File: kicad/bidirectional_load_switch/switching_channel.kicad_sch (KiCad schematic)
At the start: 17 parts, among them U201 SN74LVC1G08DCKR, U202 SN74LVC1G17DCKR, U203 UCC23313DWYR, U204 STD16N60M6, U205 STD16N60M6

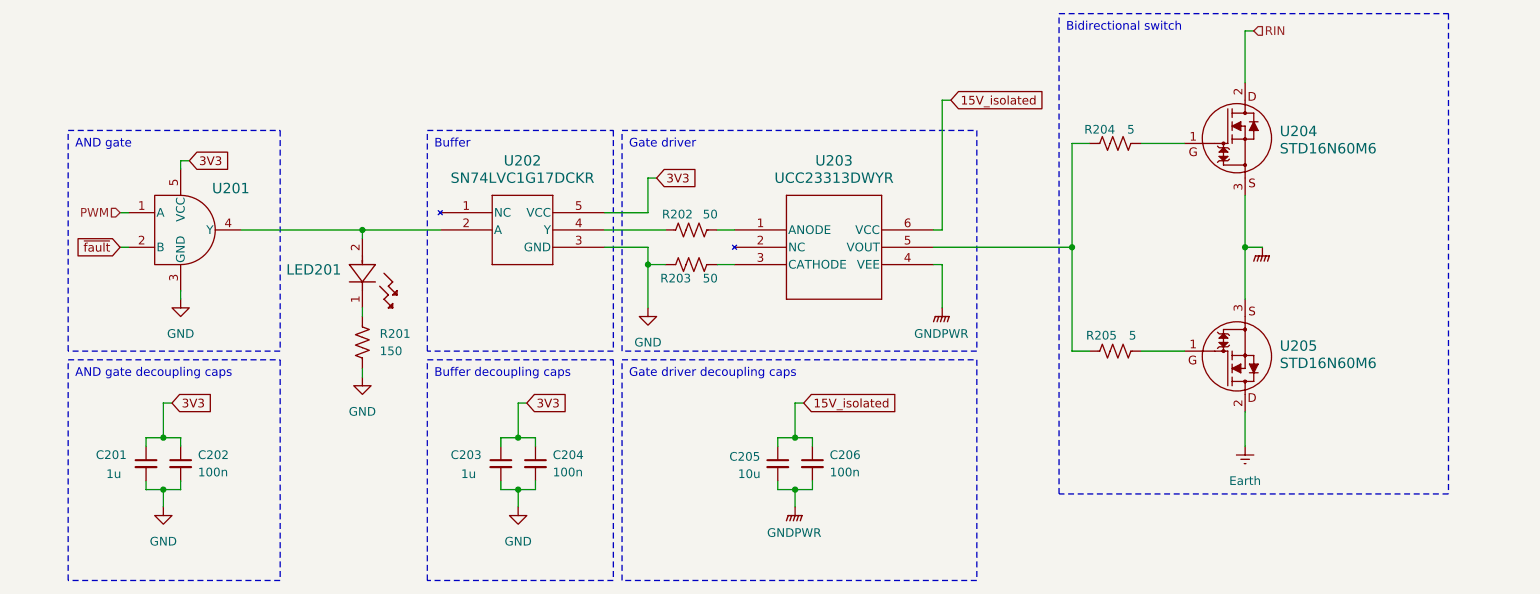
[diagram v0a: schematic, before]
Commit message: ready for order
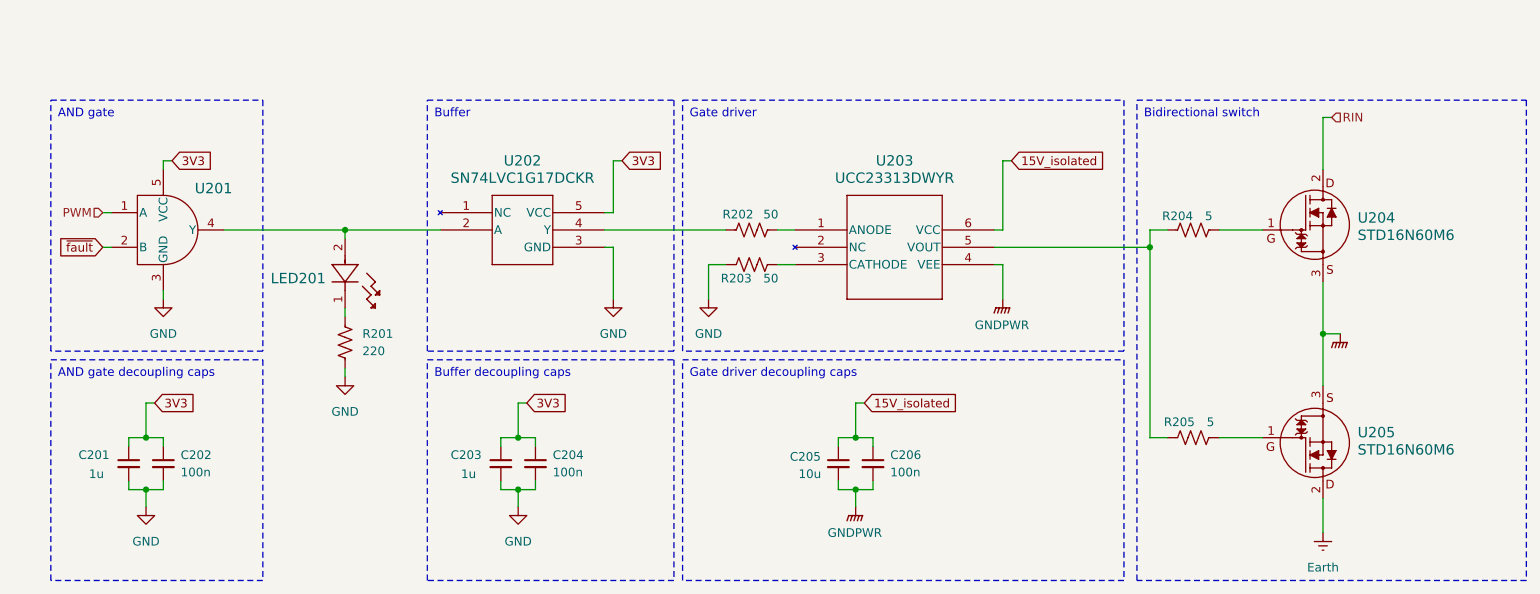
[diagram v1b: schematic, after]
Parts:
- R201: value 150 -> 220
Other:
- moved on the sheet: C201, C202, C205, C206, LED201, R201, R202, R203, R204, R205, U201, U203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
